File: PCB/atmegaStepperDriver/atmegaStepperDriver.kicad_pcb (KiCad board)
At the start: 2 copper layers, 70 parts, among them J1 Screw_Terminal_01x02, J2 Motor Output, J3 Screw_Terminal_01x02, J4 Conn_01x05_Socket, J5 Conn_01x02_Socket, Q1 TIP42C, Q10 BC547, Q11 BC557, Q12 BC547, Q13 BC557, Q14 BC547, Q15 BC557, Q16 BC547, Q2 TIP41C, Q3 TIP42C, Q4 TIP42C, Q5 TIP42C, Q6 TIP41C, Q7 TIP41C, Q8 TIP41C, Q9 BC557, U1 ATmega328P-P, U2 LM7805_TO220, Y1 Crystal

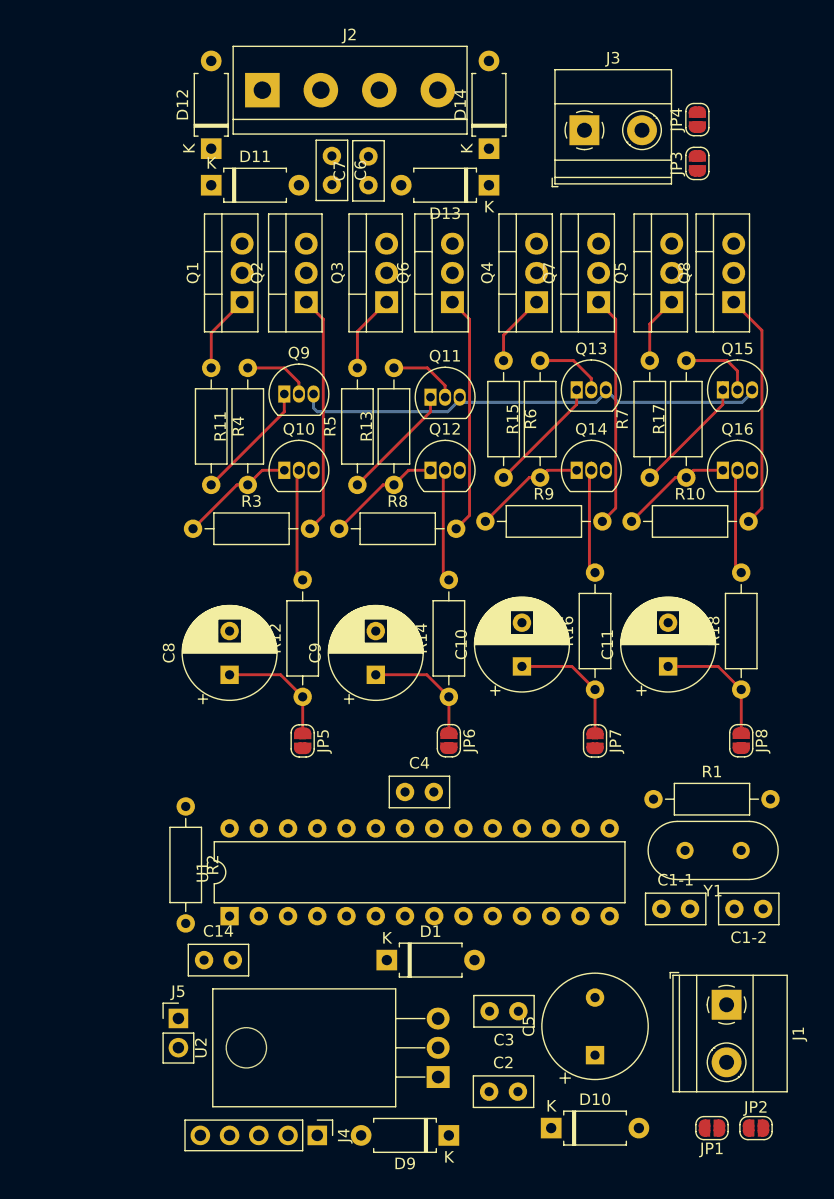
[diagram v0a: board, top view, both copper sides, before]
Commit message: communication pins;
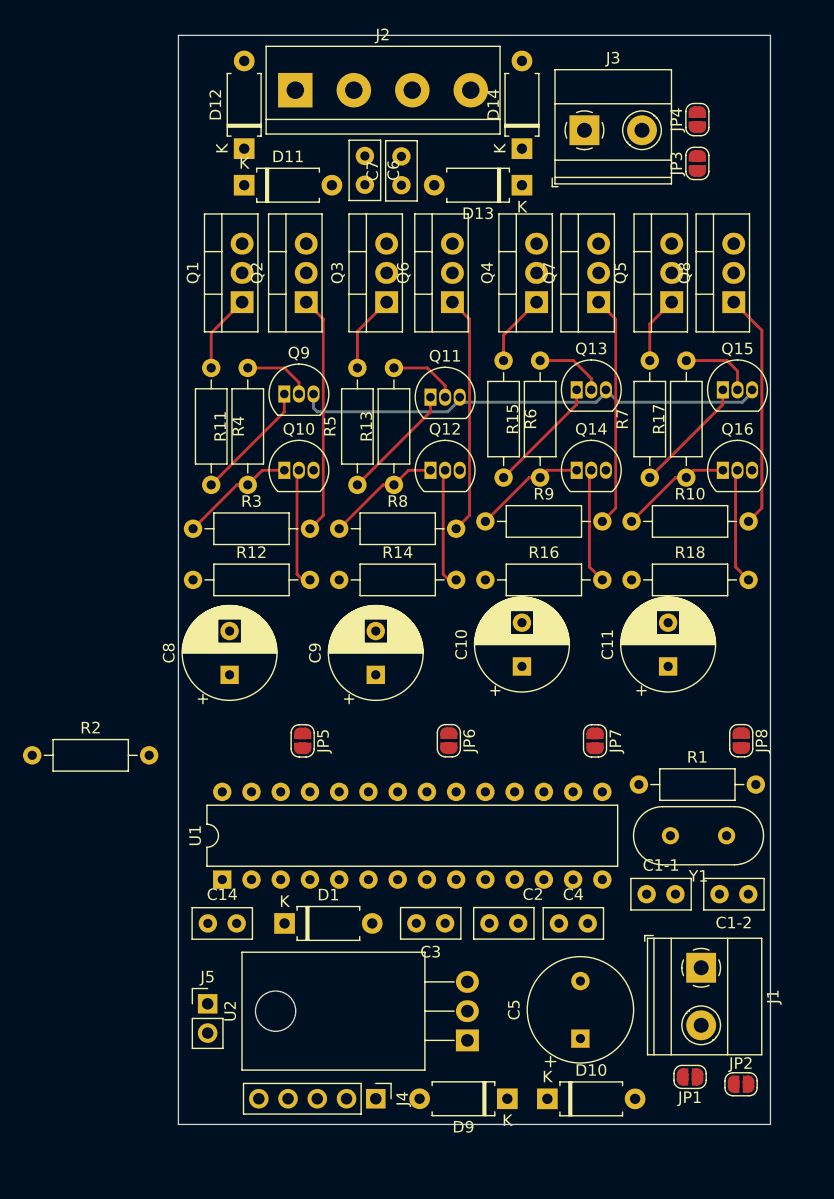
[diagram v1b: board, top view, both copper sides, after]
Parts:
- moved C4 17.6 mm to (98.5, 122.6)
- moved C2 14.6 mm to (92.4, 122.5)
- moved R2 14.1 mm to (52.7, 108.0), turned to 0 degrees
- moved R12 13.9 mm to (66.7, 92.7), turned to 0 degrees
- moved R14 13.9 mm to (79.4, 92.7), turned to 0 degrees
- moved R16 13.5 mm to (92.1, 92.7), turned to 0 degrees
- moved R18 13.5 mm to (104.8, 92.7), turned to 0 degrees
- moved C3 9.94 mm to (88.6, 122.5)
- moved D1 9.44 mm to (74.6, 122.6)
- moved D9 6.00 mm to (94.0, 137.8)
- moved J4 6.00 mm to (82.5, 137.8)
- moved JP1 4.84 mm to (109.9, 135.9)
- moved U2 4.07 mm to (90.5, 132.7)
- moved JP2 4.03 mm to (114.3, 136.5)
- moved J1 3.90 mm to (110.8, 126.4)
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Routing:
- net Gate 3: track 11.0 -> 0.00 mm
- net Gate 4: track 11.0 -> 0.00 mm
- net Gate 1: track 10.3 -> 0.00 mm
- net Gate 2: track 10.3 -> 0.00 mm
- net Net-(D1-A): track 0.90 -> 0.00 mm
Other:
- board outline added: 51.4 x 94.6 mm
- board text added: "atMega Stepper Driver Developer board V0.0.4"
- board text added: "bruh"
